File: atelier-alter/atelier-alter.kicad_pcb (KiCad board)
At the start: 2 copper layers, 81.8 x 80.3 mm, 60 parts, among them SW1 SW_DPST, SW2 SW_DPST, SW3 SW_DPST, SW4 RESET, U1 ATmega32U4-A, U2 PRTR5V0U2X, Y1 16Mhz

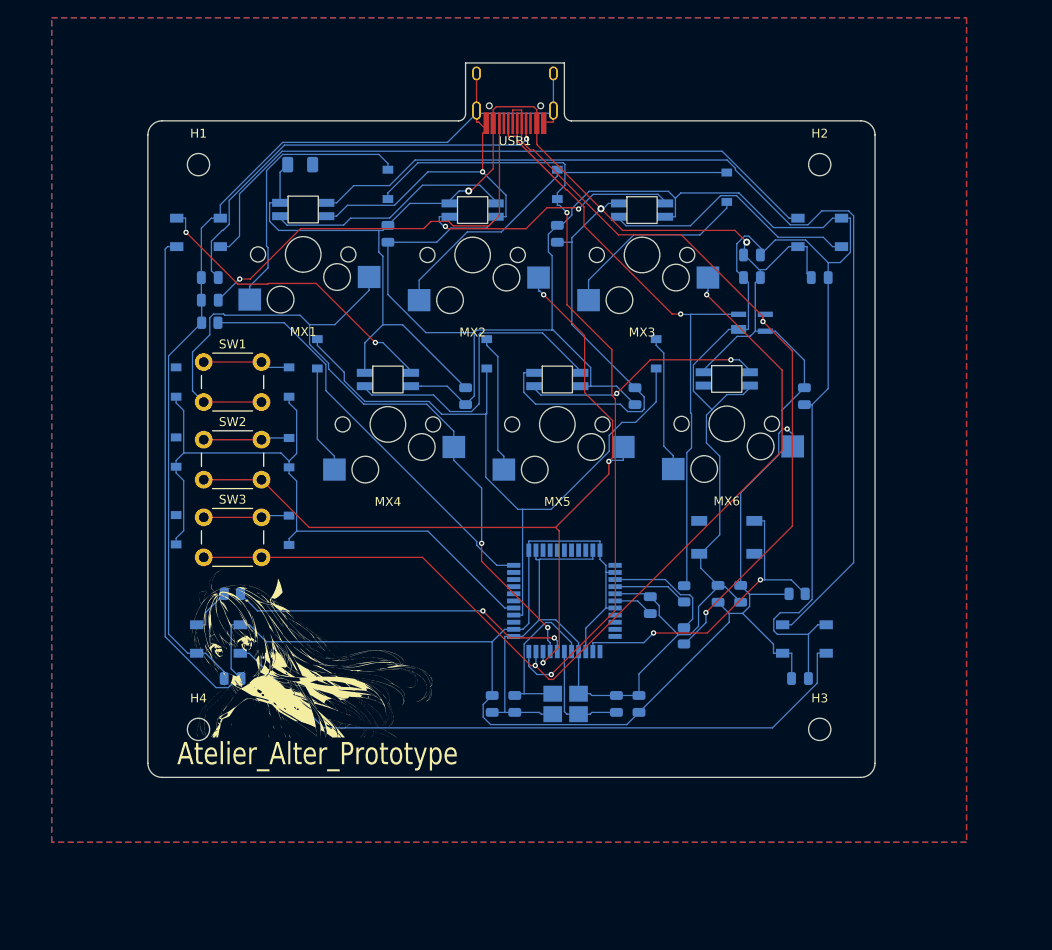
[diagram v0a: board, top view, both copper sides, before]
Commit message: rework mot chut
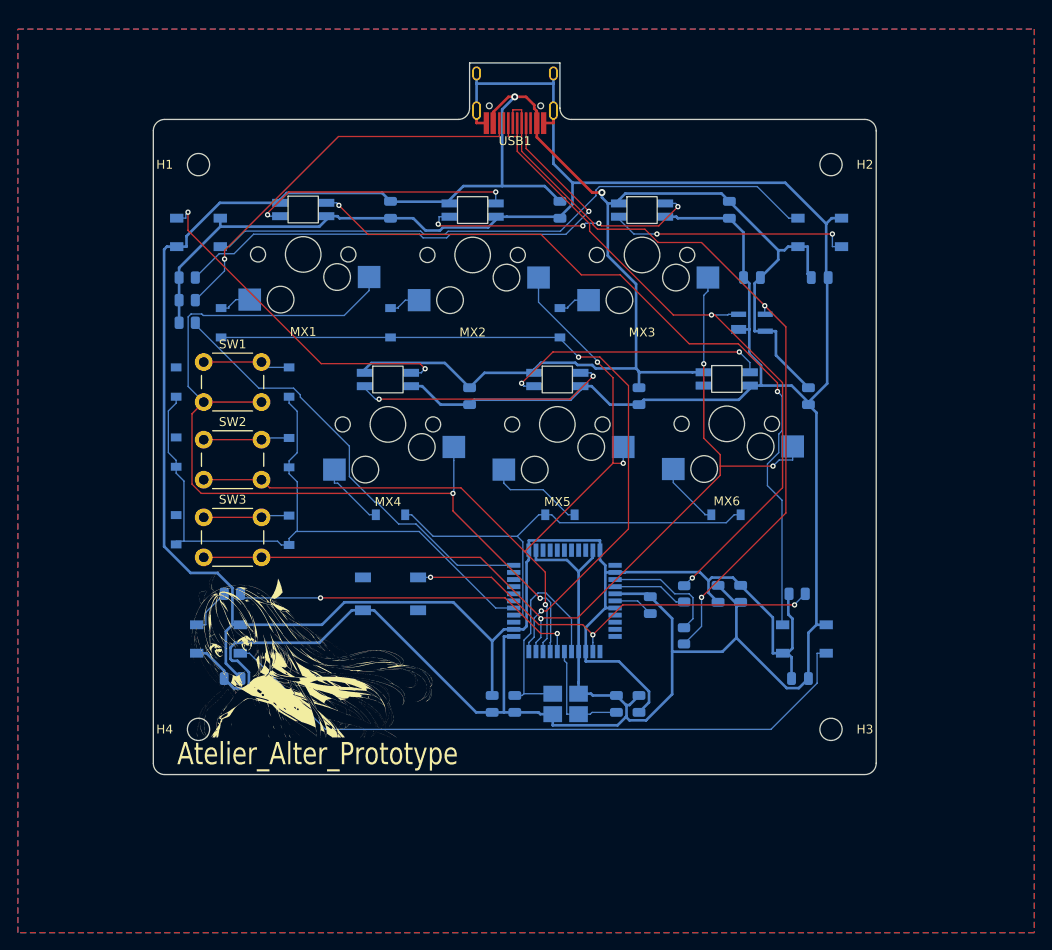
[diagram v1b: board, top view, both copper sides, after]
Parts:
- removed F1: 500mA, Fuse:Fuse_1206_3216Metric
- C12, C13, C15, C16, C8, C9: value 100uF -> 100nF
- R4, R5: footprint Capacitor_SMD:C_0805_2012Metric -> Resistor_SMD:R_0805_2012Metric
- moved SW4 38.3 mm to (143.5, 114.3)
- moved D11 24.4 mm to (124.5, 83.8)
- moved D12 24.4 mm to (143.5, 83.8)
- moved D13 24.2 mm to (162.6, 83.8), turned to 90 degrees
- moved D22 19.9 mm to (162.6, 105.4), turned to 0 degrees
- moved D21 19.9 mm to (143.5, 105.4), turned to 180 degrees
- moved D23 19.7 mm to (181.2, 105.4), turned to 180 degrees
- moved C16 5.68 mm to (181.6, 71.1), turned to 90 degrees
- moved C13 2.71 mm to (162.6, 71.1), turned to 90 degrees
- moved C9 2.71 mm to (143.5, 71.1)
- moved R4 2.54 mm to (120.7, 78.7)
- moved R5 2.54 mm to (120.7, 81.3)
- moved R6 2.54 mm to (120.7, 83.8)
- moved H2 1.27 mm to (193.0, 66.0)
- moved H3 1.27 mm to (193.0, 129.5)
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- renumbered DT11 to D14
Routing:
- net GND: track 485.0 -> 411.3 mm, vias 1 -> 0
- net +5V: track 418.9 -> 378.2 mm, vias 3 -> 2
- net ROW2: track 79.0 -> 50.6 mm
- net Net-(D11-Pad2): track 31.0 -> 3.71 mm
- net D11: track 115.2 -> 87.9 mm, vias 0 -> 2
- net ROW1: track 108.4 -> 83.1 mm
- net Net-(D12-Pad2): track 23.3 -> 3.64 mm
- net Net-(D13-Pad2): track 21.8 -> 3.64 mm
- net COL1: track 91.1 -> 107.6 mm
- net Net-(R3-Pad1): track 36.2 -> 50.0 mm, vias 2 -> 3
- net Net-(R4-Pad2): track 48.0 -> 60.5 mm
- net Net-(D23-Pad2): track 15.4 -> 7.34 mm
- net D+: track 69.6 -> 77.3 mm, vias 1 -> 2
- net Net-(C3-Pad2): track 18.2 -> 25.0 mm
- net Net-(MX4-Pad3): track 35.8 -> 29.2 mm, vias 0 -> 2
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- added copper zone on B.Cu, net GND
- added copper zone on F.Cu, net GND
- removed copper zone on B.Cu, net +5V
- removed copper zone on F.Cu, net +5V
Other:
- board size 81.8 x 80.3 mm -> 81.3 x 80 mm
